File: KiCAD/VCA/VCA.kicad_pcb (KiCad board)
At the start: 2 copper layers, 40 x 53 mm, 15 parts, among them J1 VIN, J2 VC, J3 VOUT, J4 Conn_01x03_Pin, Q1 J172, Q2 J172, U1 LT1006

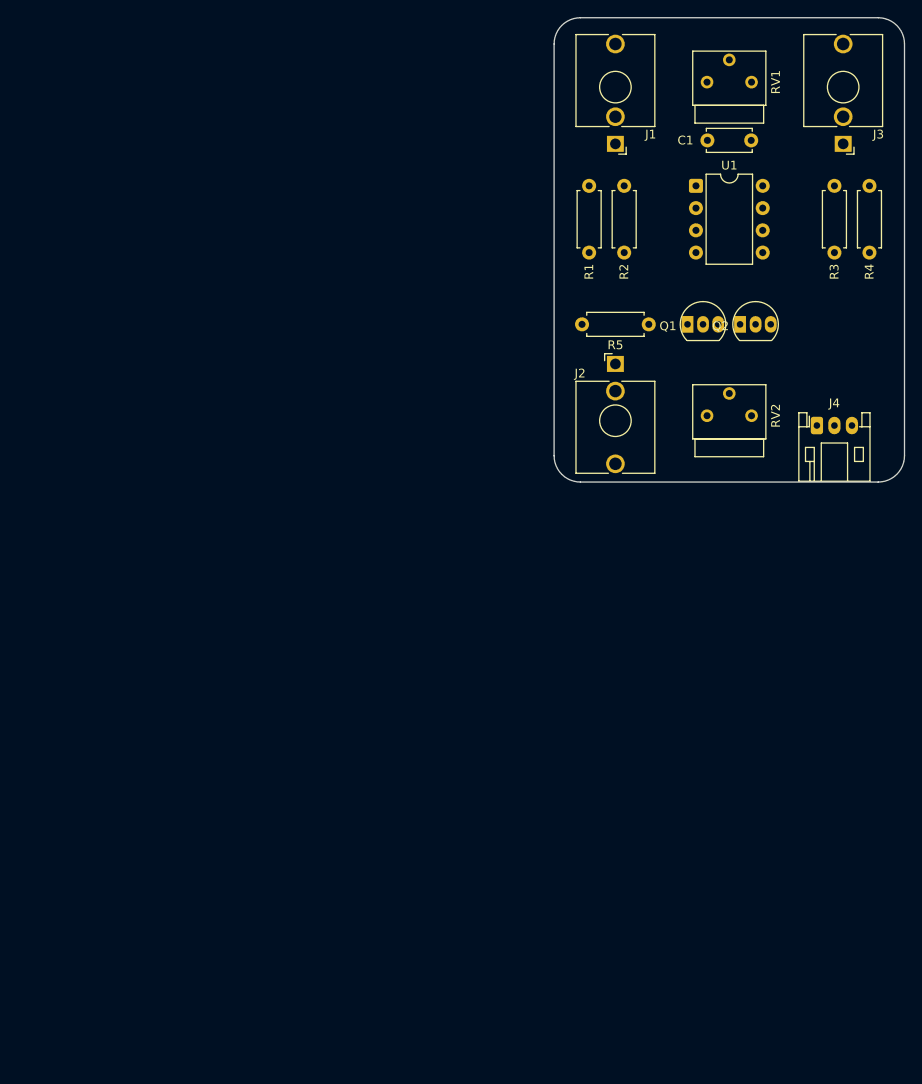
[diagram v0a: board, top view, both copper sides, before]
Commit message: VCA PCB
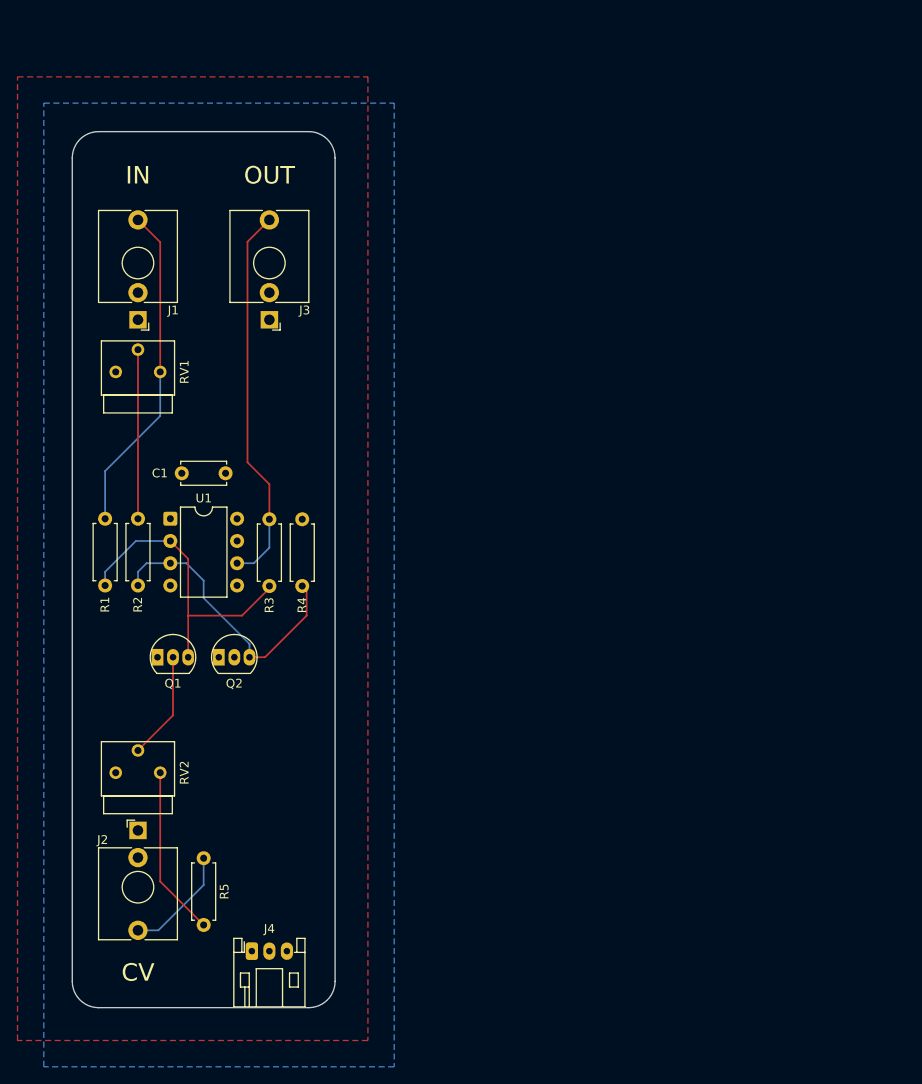
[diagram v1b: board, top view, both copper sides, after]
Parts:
- added Ref**: Val**, HackSynth:PancakeLegend Logo - 10mm, B.Cu at (137.5, 132.0)
- added Ref**: Val**, HackSynth:CCHS Logo - 10mm, B.Cu at (137.5, 120.5)
- moved J4 88.1 mm to (135.5, 143.6)
- moved R5 79.3 mm to (130.0, 132.9), turned to -90 degrees
- moved RV2 78.8 mm to (125.0, 123.2)
- moved J2 76.2 mm to (122.5, 136.2)
- moved RV1 75.2 mm to (125.0, 77.4)
- moved R4 75.1 mm to (141.2, 101.9)
- moved R3 74.9 mm to (137.5, 101.9)
- moved Q1 71.4 mm to (125.2, 110.0)
- moved C1 71.0 mm to (132.5, 89.0)
- moved U1 71.0 mm to (126.2, 94.2)
- moved Q2 70.6 mm to (132.2, 110.0)
- moved J3 68.5 mm to (137.5, 65.0)
- moved R2 67.3 mm to (122.5, 94.2)
- moved R1 67.1 mm to (118.8, 94.2)
- moved J1 58.1 mm to (122.5, 65.0)
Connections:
- J1 pad S: unconnected-(J1-PadS) -> GND
- J2 pad S: unconnected-(J2-PadS) -> GND
- J3 pad S: unconnected-(J3-PadS) -> GND
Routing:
- net Net-(J3-PadT): track 0.00 -> 43.9 mm
- net Net-(J1-PadT): track 0.00 -> 37.8 mm
- net Net-(Q1-D): track 0.00 -> 35.5 mm
- net Net-(Q2-D): track 0.00 -> 33.1 mm
- net Net-(R5-Pad2): track 0.00 -> 19.4 mm
- net Net-(R2-Pad1): track 0.00 -> 19.3 mm
- net Net-(J2-PadT): track 0.00 -> 12.9 mm
- net Net-(Q1-G): track 0.00 -> 12.3 mm
- added copper zone on B.Cu, net GND
- added copper zone on F.Cu, net GND
- added copper zone on In1.Cu, net VDD
- added copper zone on In2.Cu, net VSS
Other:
- board size 40 x 53 mm -> 30 x 100 mm
- copper layers 2 -> 4
- board text added: "CV"
- board text added: "IN"
- board text added: "OUT"
- board text added: "VCA v1-0 - PancakeLegend 2025"
